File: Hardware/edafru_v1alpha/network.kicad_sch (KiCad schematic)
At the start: 9 parts, among them U6 SN65HVD1050D

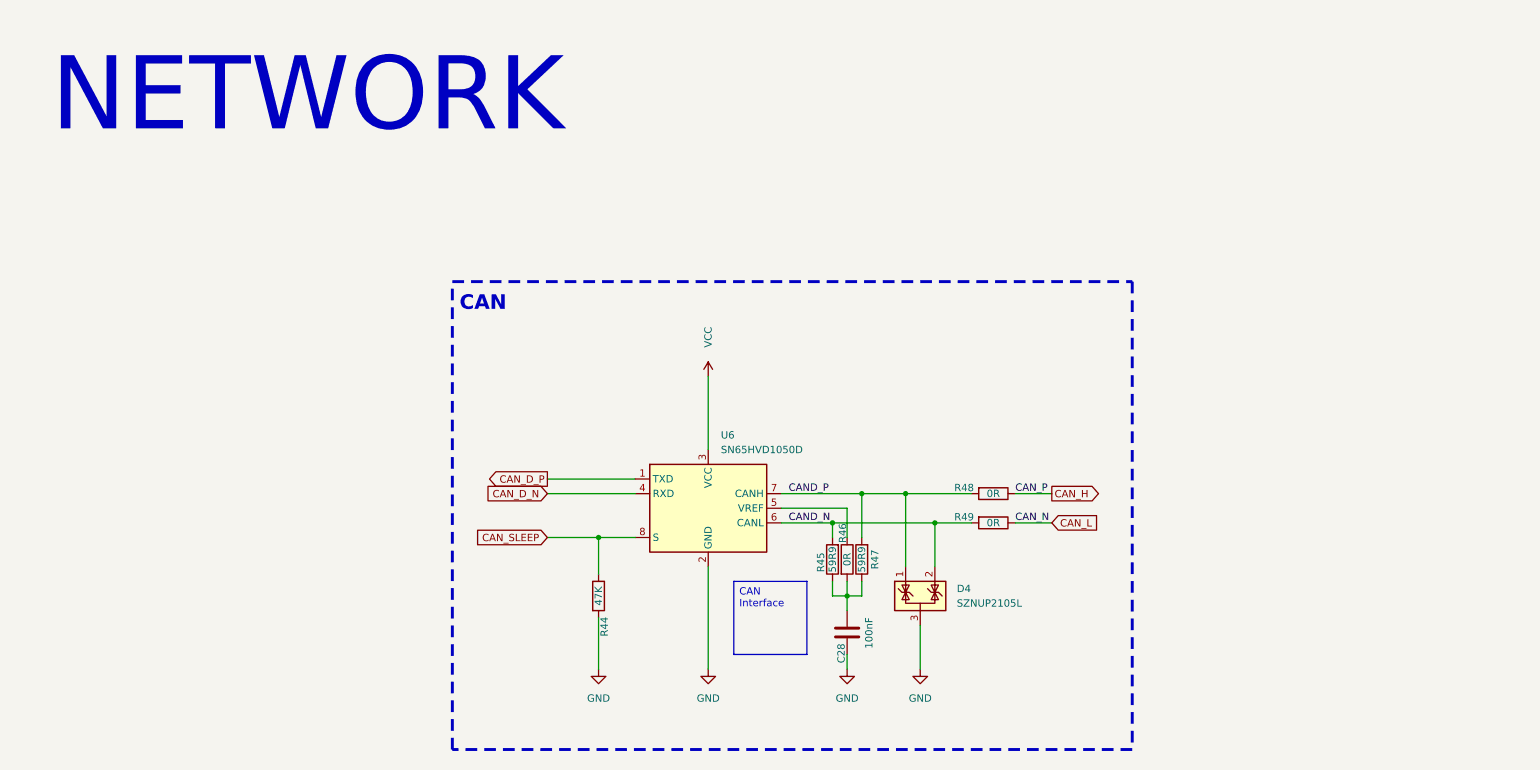
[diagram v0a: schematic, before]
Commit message: PCB is developing...
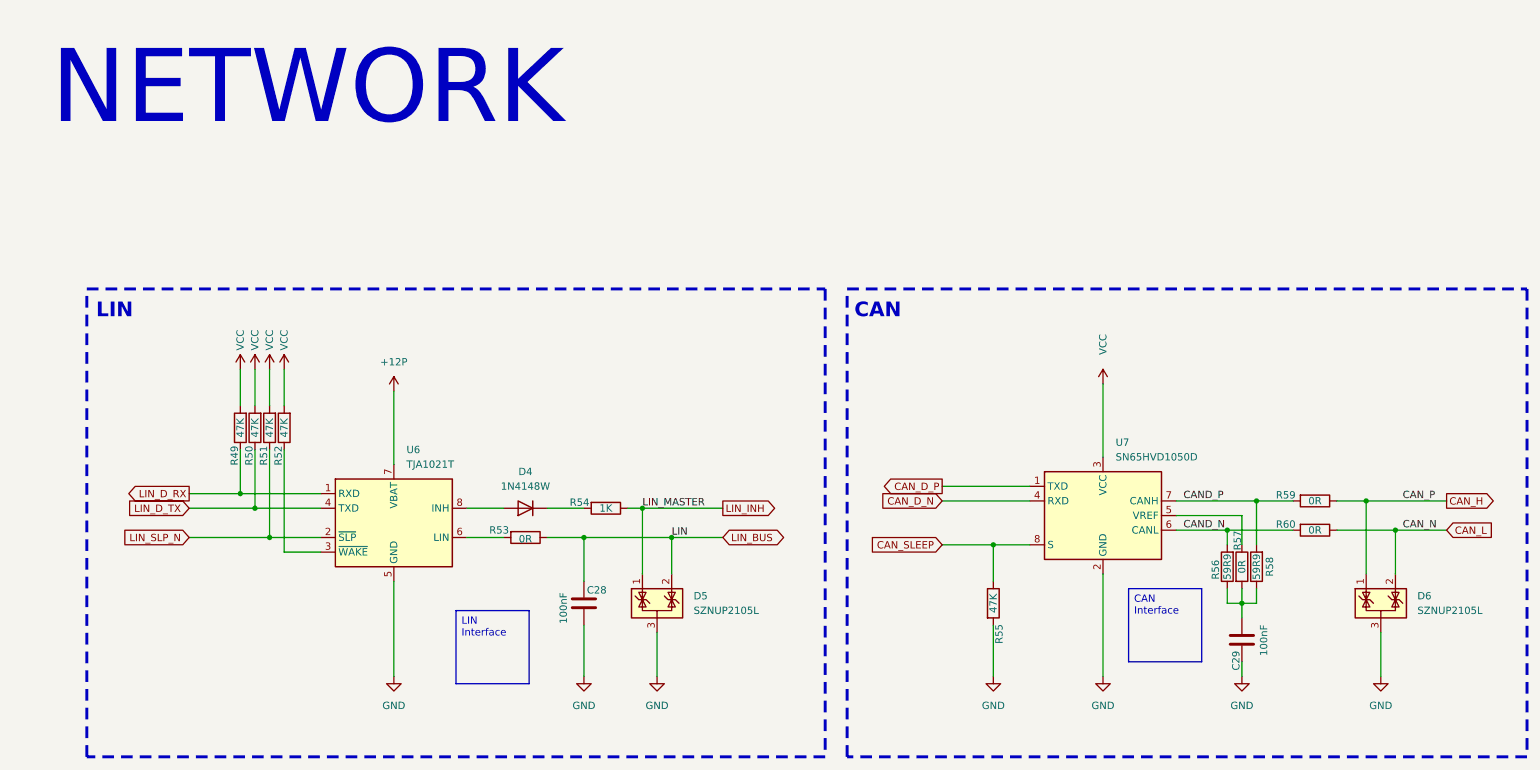
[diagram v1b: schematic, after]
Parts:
- removed D4: SZNUP2105L, Package_TO_SOT_SMD:SOT-23, symbol Power_Protection:SZNUP2105L
- removed R44: 47K, Resistor_SMD:R_0603_1608Metric_Pad0.98x0.95mm_HandSolder, symbol Device:R
- removed R45, R47: 59R9, Resistor_SMD:R_0603_1608Metric_Pad0.98x0.95mm_HandSolder, symbol Device:R
- removed R46, R48: 0R, Resistor_SMD:R_0603_1608Metric_Pad0.98x0.95mm_HandSolder, symbol Device:R
- removed U6: SN65HVD1050D, Package_SO:SOIC-8_3.9x4.9mm_P1.27mm, symbol Interface_CAN_LIN:SN65HVD1050D
- added C29: 100nF, Capacitor_SMD:C_0603_1608Metric_Pad1.08x0.95mm_HandSolder, symbol Device:C
- added D4: 1N4148W, Diode_SMD:D_SOD-123, symbol Diode:1N4148W
- added D5, D6: SZNUP2105L, Package_TO_SOT_SMD:SOT-23, symbol Power_Protection:SZNUP2105L
- added R50, R51, R52, R55: 47K, Resistor_SMD:R_0603_1608Metric_Pad0.98x0.95mm_HandSolder, symbol Device:R
- added R53, R57, R59, R60: 0R, Resistor_SMD:R_0603_1608Metric_Pad0.98x0.95mm_HandSolder, symbol Device:R
- added R54: 1K, Resistor_SMD:R_0603_1608Metric_Pad0.98x0.95mm_HandSolder, symbol Device:R
- added R56, R58: 59R9, Resistor_SMD:R_0603_1608Metric_Pad0.98x0.95mm_HandSolder, symbol Device:R
- added U6: TJA1021T, Package_SO:SOIC-8_3.9x4.9mm_P1.27mm, symbol Interface_CAN_LIN:TJA1021T
- added U7: SN65HVD1050D, Package_SO:SOIC-8_3.9x4.9mm_P1.27mm, symbol Interface_CAN_LIN:SN65HVD1050D
- R49: value 0R -> 47K
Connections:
- net CAND_N: now also R56.2, R60.2, U7.6 (CANL); no longer R49.2
- net CAND_P: now also R58.2, R59.2, U7.7 (CANH)
- net CAN_D_N: now also U7.4 (RXD)
- net CAN_D_P: now also U7.1 (TXD)
- net CAN_H: now also D6.1 (K), R59.1
- net CAN_L: now also D6.2 (K), R60.1; no longer R49.1
- net CAN_SLEEP: now also R55.1, U7.8 (S)
- net GND: now also C29.2, D5.3 (A), D6.3 (A), R55.2, U6.5 (GND), U7.2 (GND)
- net VCC: now also R49.2, R50.2, R51.2, R52.2, U7.3 (VCC)
- net LIN_BUS: now reaches C28.1
- net LIN_BUS: now also D5.2 (K), R53.1
- new net: R53.2, U6.6 (LIN)
- new net: D4.1 (K), R54.2
- new net: R57.1, U7.5 (VREF)
- new net: C29.1, R56.1, R57.2, R58.1
- new net: R52.1, U6.3 (~{WAKE})
- new net: D4.2 (A), U6.8 (INH)
- new net +12P: U6.7 (VBAT)
- new net LIN_D_RX: R49.1, U6.1 (RXD)
- new net LIN_D_TX: R50.1, U6.4 (TXD)
- new net LIN_INH: D5.1 (K), R54.1
- new net LIN_SLP_N: R51.1, U6.2 (~{SLP})
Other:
- note added: "LIN"
